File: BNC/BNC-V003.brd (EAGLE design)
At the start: 100 x 80 mm, 23 parts, among them IC1 LM339N, IC2 74AC08N, J1 POWER_JACKSLT

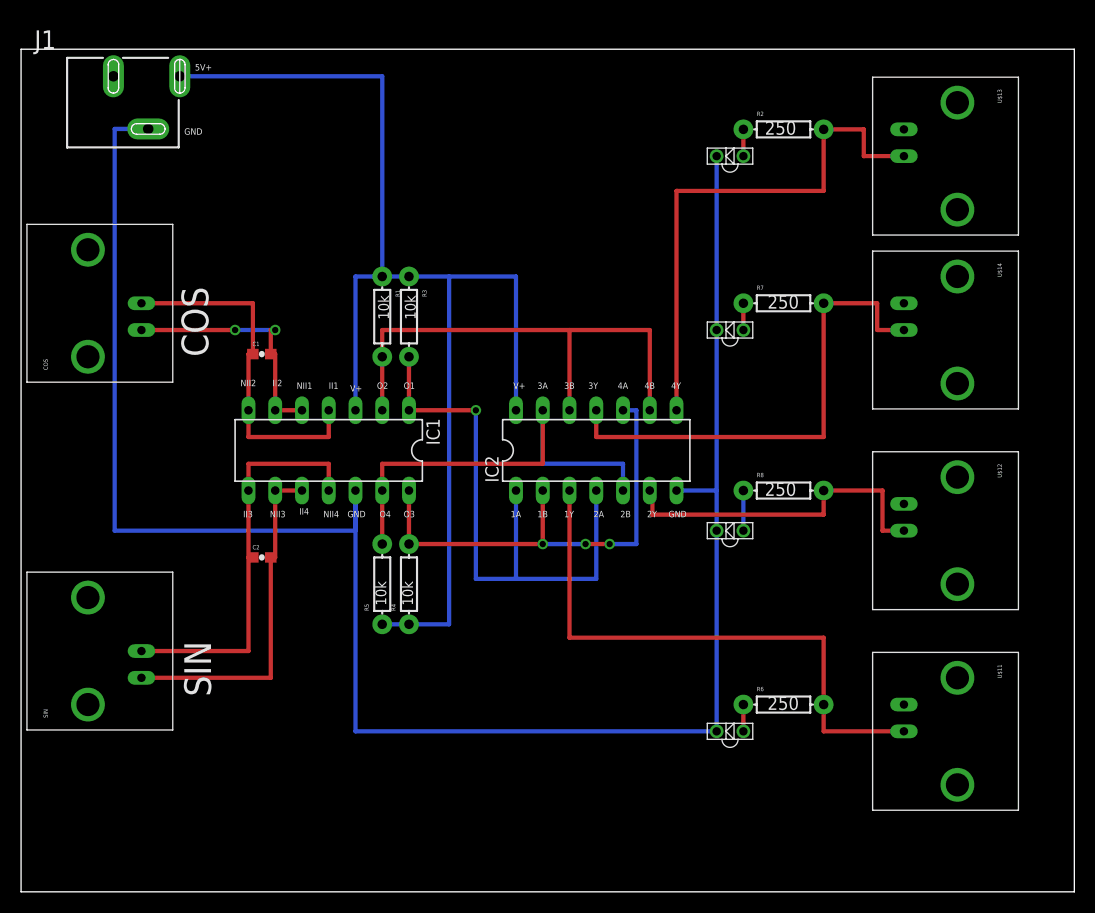
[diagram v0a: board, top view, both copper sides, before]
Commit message: yyyyyyyy enter the commit message for your changes. Lines starting
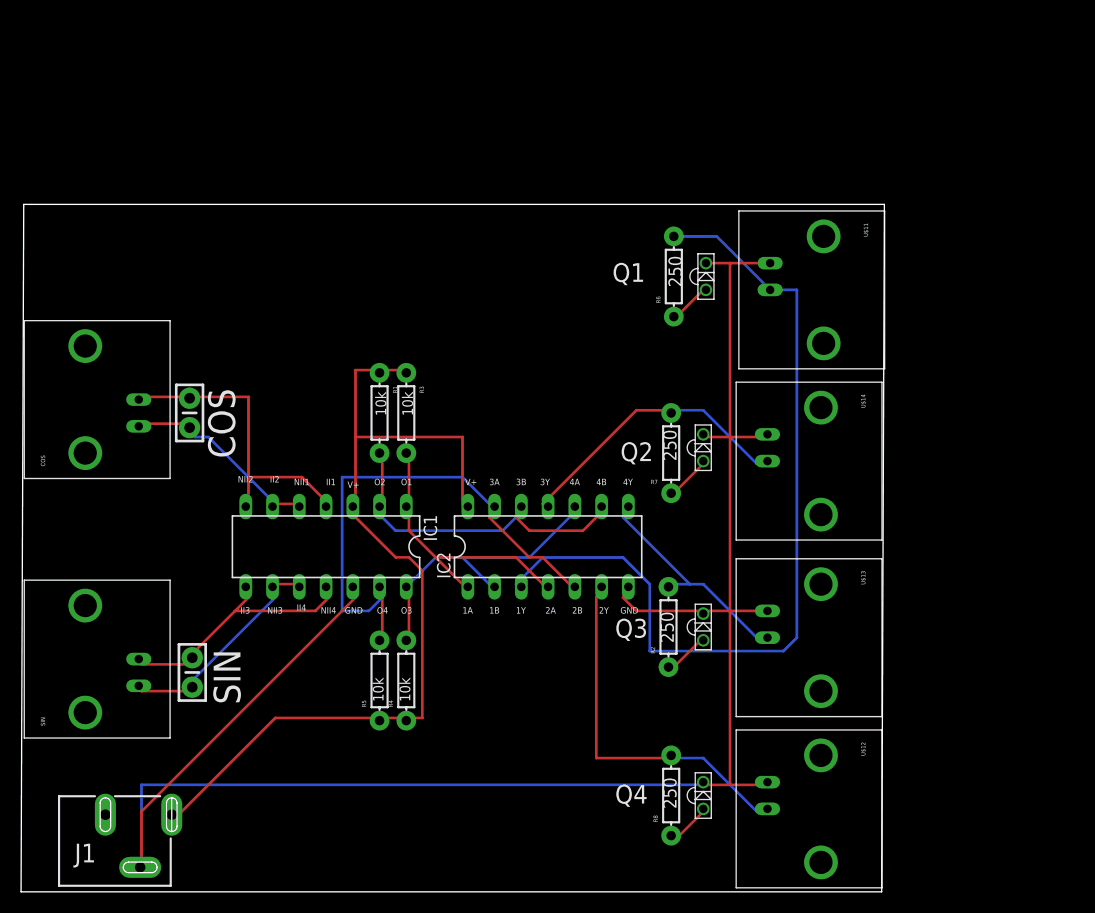
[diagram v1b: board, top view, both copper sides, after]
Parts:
- removed C2: 0.1uF, SparkFun-Capacitors:0603-CAP
- added C3: (no value), SparkFun-Capacitors:CAP-PTH-SMALL-KIT
- C1: value 0.1uF -> (none); device SparkFun-Capacitors:0603-CAP -> SparkFun-Capacitors:CAP-PTH-SMALL-KIT
- moved J1 70.1 mm to (0.51, 9.91)
- moved R2 48.5 mm to (61.5, 25.1), turned to 90 degrees
- moved U$13 47.5 mm to (70.9, 24.1)
- moved IAG3-D3 44.8 mm to (64.8, 25.1), turned to 270 degrees
- moved U$11 43.8 mm to (71.1, 57.1)
- moved IAG-D1 43.2 mm to (65.0, 58.4), turned to 270 degrees
- moved R6 42.0 mm to (62.0, 58.4), turned to 90 degrees
- moved C1 30.9 mm to (16.3, 20.8), turned to 270 degrees
- moved R8 30.9 mm to (61.7, 9.14), turned to 90 degrees
- moved U$12 29.4 mm to (70.9, 7.87)
- moved IAG2-D2 25.3 mm to (64.8, 9.14), turned to 270 degrees
- moved U$14 18.0 mm to (70.9, 40.9)
- moved R7 17.8 mm to (61.7, 41.7), turned to 90 degrees
- moved IAG4-D4 11.5 mm to (64.8, 42.2), turned to 270 degrees
- moved IC2 10.2 mm to (50.0, 32.8)
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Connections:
- net GND: now also U$11.GND, U$12.GND, U$13.GND, U$14.GND
- net N$11: now also C1.2; no longer C2.2
- net N$7: now also C3.2; no longer C1.2
- net N$8: now also C3.1; no longer C1.1
- net N$9: now also C1.1; no longer C2.1
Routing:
- net 5V: track 118.2 -> 87.6 mm
- net N$12: track 50.8 -> 21.7 mm
- net N$16: track 54.9 -> 83.0 mm
- net N$4: track 55.6 -> 27.6 mm, vias 1 -> 0
- net N$2: track 47.0 -> 27.8 mm
- net N$5: track 45.7 -> 28.7 mm, vias 3 -> 0
- net N$1: track 48.3 -> 32.7 mm
- net N$9: track 38.5 -> 25.7 mm
- net N$11: track 33.0 -> 22.1 mm
- net N$6: track 43.2 -> 50.8 mm
- net N$7: track 23.7 -> 19.9 mm, vias 2 -> 0
- net N$8: track 33.9 -> 30.1 mm
- net N$14: track 32.5 -> 34.9 mm
- net N$13: track 2.54 -> 4.65 mm
- net N$3: track 2.54 -> 4.41 mm
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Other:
- board size 100 x 80 mm -> 82 x 65.3 mm
- board text added: "Q1"
- board text added: "Q2"
- board text added: "Q3"
- board text added: "Q4"
- board text removed: "5V+"
